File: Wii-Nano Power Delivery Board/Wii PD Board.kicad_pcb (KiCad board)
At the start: 2 copper layers, 31.5 x 16.2 mm, 11 parts, among them J1 USB4105-GF-A, Q1 DMG3406L, U1 IP2721

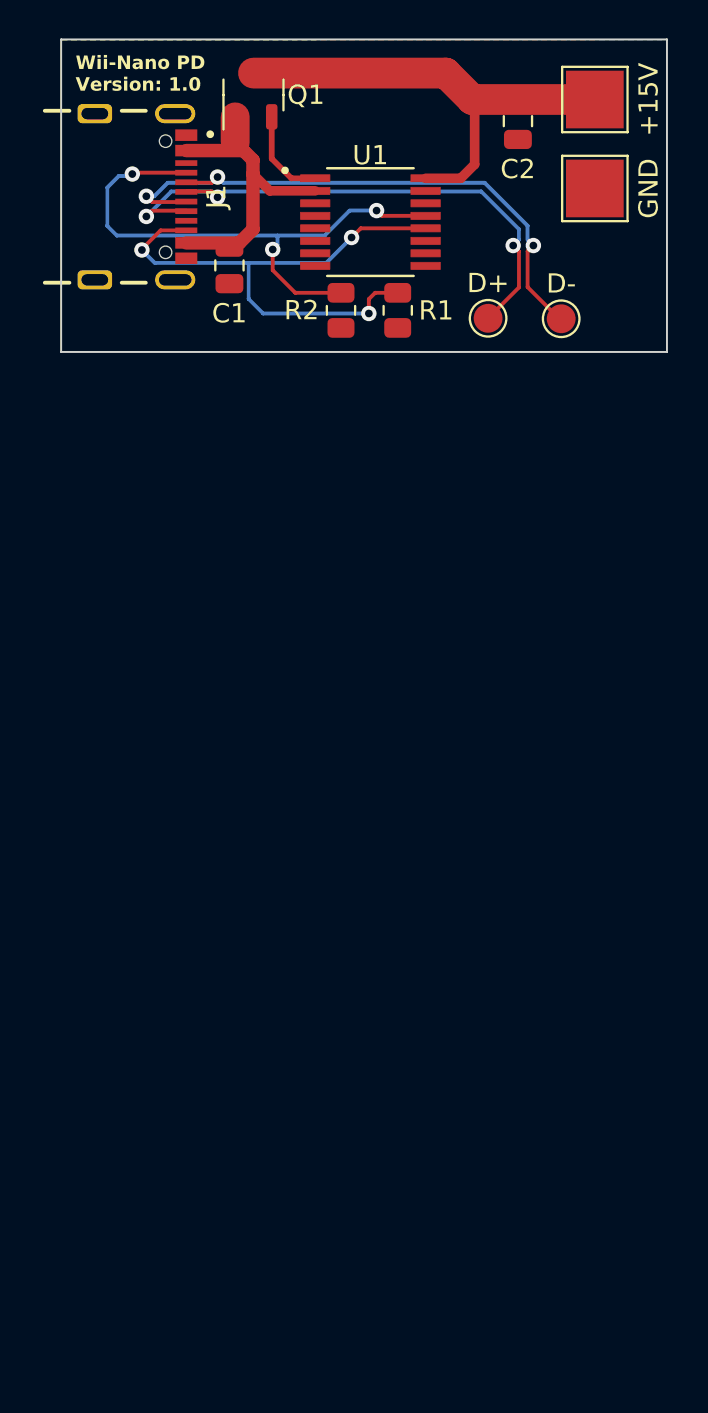
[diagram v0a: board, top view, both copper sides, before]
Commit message: Add files via upload
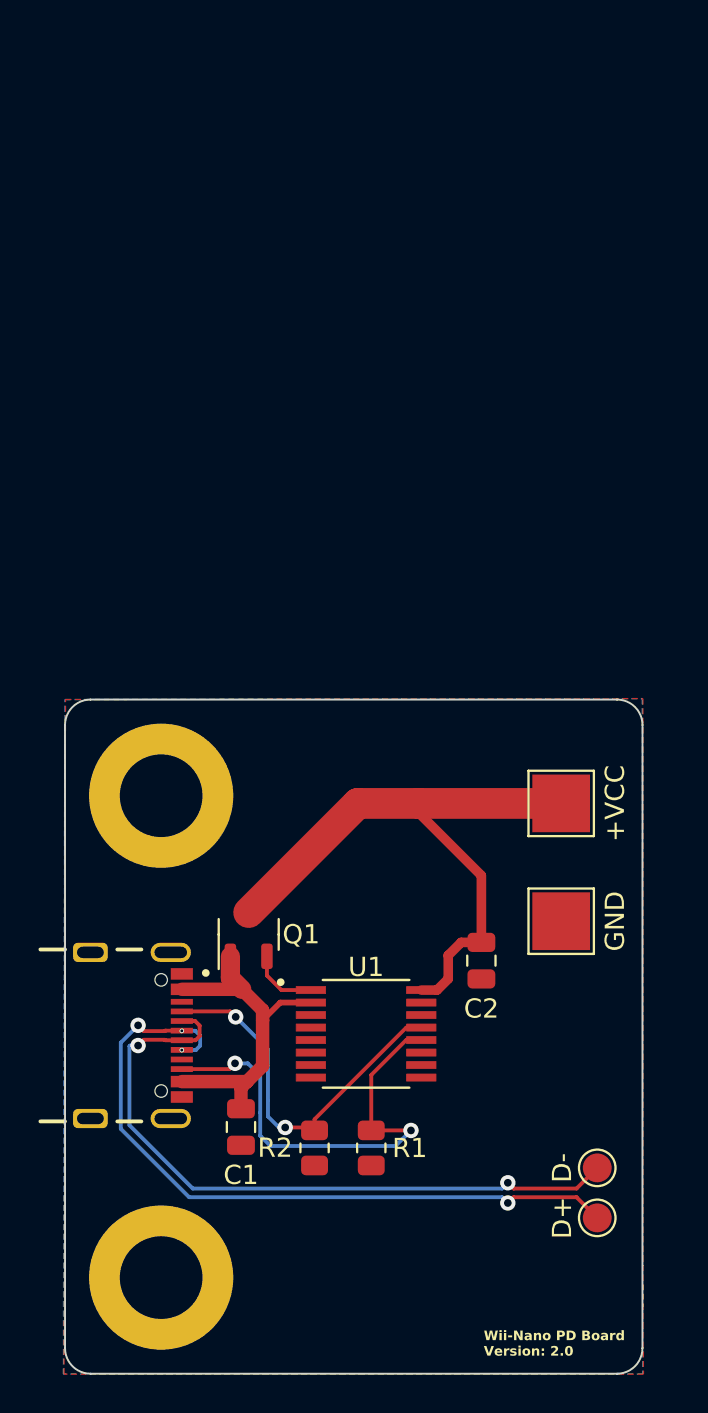
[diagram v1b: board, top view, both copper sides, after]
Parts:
- added REF**: MountingHole_4.3mm_M4_DIN965_Pad, MountingHole:MountingHole_4.3mm_M4_DIN965_Pad, F.Cu at (34.2, 77.3)
- added REF**: MountingHole_4.3mm_M4_DIN965_Pad, MountingHole:MountingHole_4.3mm_M4_DIN965_Pad, F.Cu at (34.2, 102.4)
- moved D+ 47.1 mm to (56.9, 99.3), turned to 0 degrees
- moved C1 44.8 mm to (38.4, 94.5)
- moved D- 44.2 mm to (56.9, 96.7), turned to 0 degrees
- moved C2 43.7 mm to (50.9, 85.9)
- moved Q1 43.7 mm to (38.8, 84.5)
- moved J1 43.6 mm to (30.5, 89.8)
- moved R1 43.6 mm to (45.1, 95.6)
- moved R2 43.6 mm to (42.2, 95.6)
- moved U1 42.2 mm to (44.9, 89.7)
- moved GND 38.1 mm to (55.0, 83.8)
- moved +VCC 36.6 mm to (55.0, 77.7)
- renumbered +15V to +VCC
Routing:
- net Net-(J1-CC1): track 29.8 -> 19.6 mm, vias 3 -> 2
- net +15VOUT: track 24.6 -> 32.0 mm
- net /D+: track 30.5 -> 37.8 mm, vias 3 -> 4
- net Net-(J1-CC2): track 29.4 -> 24.3 mm, vias 3 -> 2
- net /D-: track 31.0 -> 36.0 mm, vias 3 -> 2
- net VBUS: track 16.0 -> 18.5 mm
- net Net-(Q1-G): track 4.86 -> 3.60 mm
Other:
- board size 31.5 x 16.2 mm -> 30 x 35.1 mm
- board text added: "Wii-Nano PD Board Version: 2.0"
- board text removed: "Wii-Nano PD Version: 1.0"
